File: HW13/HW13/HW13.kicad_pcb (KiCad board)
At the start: 2 copper layers, 39 parts, among them J1 Barrel_Jack_MountingPin, U1 LM7805_TO220, U2 MC34063AP, U3 NE555P, U4 SC39-11SRWA, U5 SC39-11SRWA, U6 CD4026B, U7 CD4026B

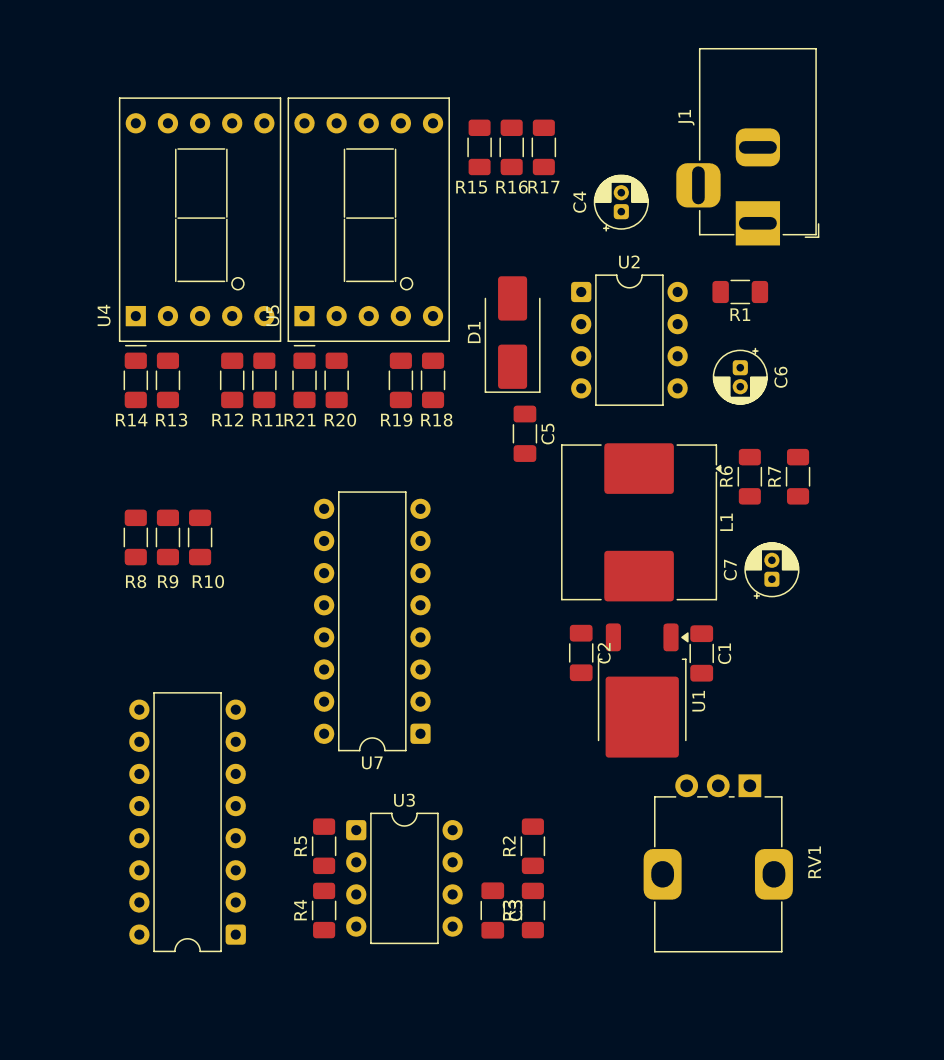
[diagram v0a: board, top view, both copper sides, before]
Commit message: HW13 PCB done
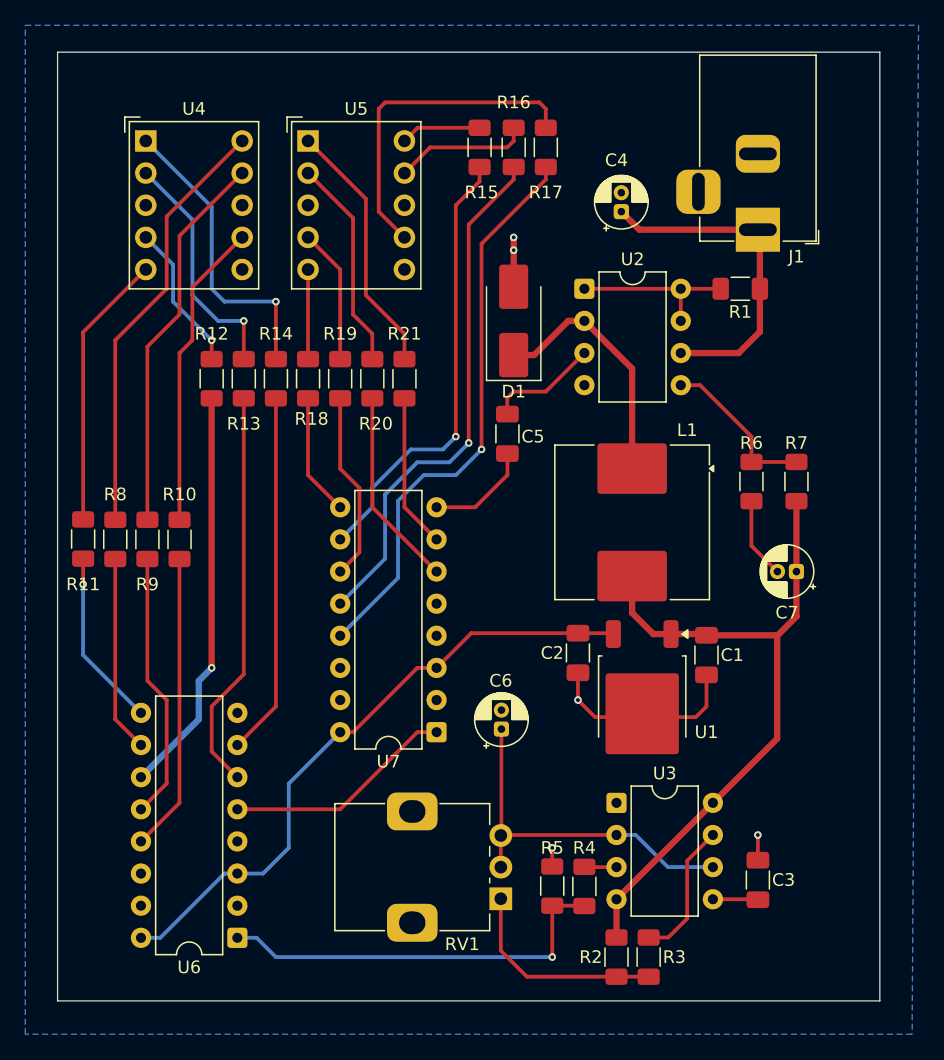
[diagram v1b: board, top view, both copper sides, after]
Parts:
- R7: value 6k2 -> 6k8
- U4, U5: footprint Display_7Segment:D1X8K -> Display_7Segment:Sx39-1xxxxx
- moved C6 34.2 mm to (71.2, 132.3), turned to 90 degrees
- moved RV1 21.6 mm to (71.1, 145.8), turned to 180 degrees
- moved C3 21.1 mm to (91.4, 144.3)
- moved U3 20.7 mm to (80.3, 138.2)
- moved R4 20.7 mm to (77.7, 144.8), turned to -90 degrees
- moved R11 19.0 mm to (38.1, 117.3)
- moved R5 18.3 mm to (75.2, 144.8)
- moved U4 13.9 mm to (43.1, 85.9), turned to 0 degrees
- moved U5 13.8 mm to (55.9, 85.9), turned to 0 degrees
- moved R14 11.1 mm to (53.3, 104.6)
- moved R2 11.0 mm to (80.3, 150.4)
- moved R18 9.88 mm to (55.9, 104.6)
- moved R3 9.86 mm to (82.8, 150.4), turned to -90 degrees
- moved R21 7.90 mm to (63.5, 104.6)
- moved R13 6.00 mm to (50.8, 104.6)
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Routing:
- net +10V: track 0.00 -> 56.0 mm
- net +5V: track 0.00 -> 50.2 mm
- net Net-(U7-C): track 0.00 -> 45.3 mm, vias 0 -> 1
- net Net-(U7-B): track 0.00 -> 41.7 mm, vias 0 -> 1
- net GND: track 0.00 -> 38.4 mm, vias 0 -> 5
- net Net-(U7-A): track 0.00 -> 35.5 mm, vias 0 -> 1
- net Net-(U4-A): track 0.00 -> 34.1 mm
- net Net-(U6-E): track 0.00 -> 32.3 mm, vias 0 -> 1
- net P-P: track 0.00 -> 32.1 mm, vias 0 -> 1
- net Net-(U6-F): track 0.00 -> 31.8 mm
- net Net-(U4-B): track 0.00 -> 30.5 mm
- net Net-(U3-THRES): track 0.00 -> 29.0 mm
- net Net-(U6-G): track 0.00 -> 28.7 mm
- net +12V: track 0.00 -> 27.0 mm
- net Net-(U5-C): track 0.00 -> 26.1 mm
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- added copper zone on B.Cu, net GND
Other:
- board outline added: 65 x 75 mm
- board text removed: "${REFERENCE}"
